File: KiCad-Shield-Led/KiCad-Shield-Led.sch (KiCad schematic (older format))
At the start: 16 parts, among them P1 Power, P2 Analog, P3 Digital, P4 Digital, P5 CONN_01X01, P6 CONN_01X01, P7 CONN_01X01, P8 CONN_01X01

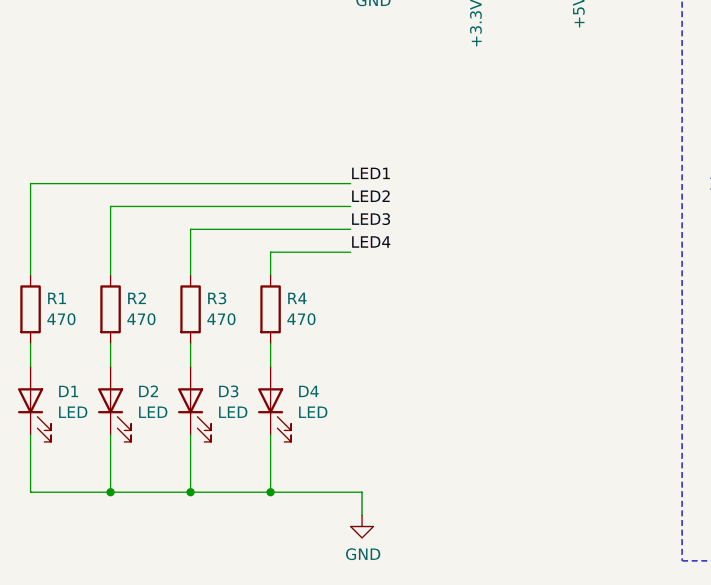
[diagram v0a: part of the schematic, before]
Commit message: Generation de la Netlist
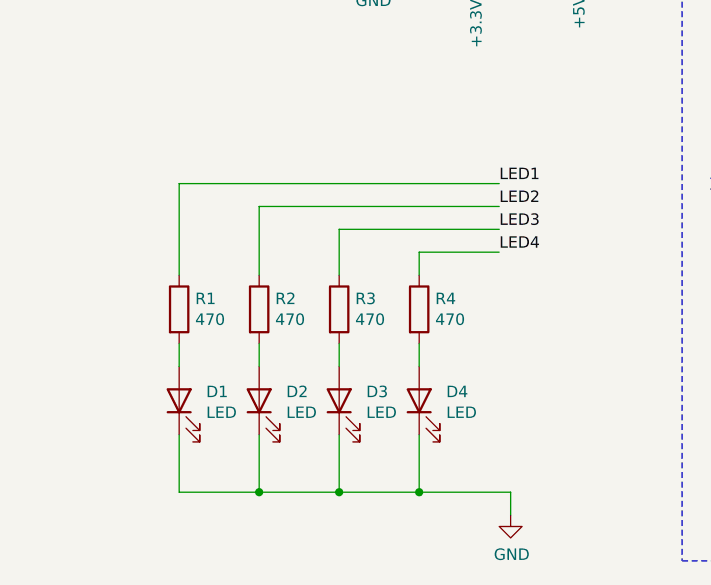
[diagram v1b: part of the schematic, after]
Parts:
- D1, D2, D3, D4: footprint (none) -> LED_THT:LED_D5.0mm
- R1, R2, R3, R4: footprint (none) -> Resistor_THT:R_Axial_DIN0207_L6.3mm_D2.5mm_P10.16mm_Horizontal
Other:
- moved on the sheet: D1, D2, D3, D4, R1, R2, R3, R4
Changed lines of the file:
@@
 L Device:LED D1
 U 1 1 5FC4CFF8
-P 5650 2750
-F 0 "D1" V 5689 2632 50  0000 R CNN
-F 1 "LED" V 5598 2632 50  0000 R CNN
-F 2 "" H 5650 2750 50  0001 C CNN
-F 3 "~" H 5650 2750 50  0001 C CNN
-	1    5650 2750
+P 6300 2750
+F 0 "D1" V 6339 2632 50  0000 R CNN
+F 1 "LED" V 6248 2632 50  0000 R CNN
+F 2 "LED_THT:LED_D5.0mm" H 6300 2750 50  0001 C CNN
+F 3 "~" H 6300 2750 50  0001 C CNN
+	1    6300 2750
 	0    -1   -1   0
 $EndComp
@@
 L Device:R R1
 U 1 1 5FC4E899
-P 5650 2350
-F 0 "R1" H 5720 2396 50  0000 L CNN
-F 1 "470" H 5720 2305 50  0000 L CNN
-F 2 "" V 5580 2350 50  0001 C CNN
-F 3 "~" H 5650 2350 50  0001 C CNN
-	1    5650 2350
+P 6300 2350
+F 0 "R1" H 6370 2396 50  0000 L CNN
+F 1 "470" H 6370 2305 50  0000 L CNN
+F 2 "Resistor_THT:R_Axial_DIN0207_L6.3mm_D2.5mm_P10.16mm_Horizontal" V 6230 2350 50  0001 C CNN
+F 3 "~" H 6300 2350 50  0001 C CNN
+	1    6300 2350
 	1    0    0    -1
 $EndComp
 Wire Wire Line
-	5650 2500 5650 2600
+	6300 2500 6300 2600
 Wire Wire Line
-	5650 2900 5650 3150
+	6300 2900 6300 3150
 Wire Wire Line
-	5650 3150 6000 3150
+	6300 3150 6650 3150
 Wire Wire Line
-	7100 3150 7100 3250
+	7750 3150 7750 3250
 $Comp
 L Device:LED D2
 U 1 1 5FC5721B
-P 6000 2750
-F 0 "D2" V 6039 2632 50  0000 R CNN
-F 1 "LED" V 5948 2632 50  0000 R CNN
-F 2 "" H 6000 2750 50  0001 C CNN
-F 3 "~" H 6000 2750 50  0001 C CNN
-	1    6000 2750
+P 6650 2750
+F 0 "D2" V 6689 2632 50  0000 R CNN
+F 1 "LED" V 6598 2632 50  0000 R CNN
+F 2 "LED_THT:LED_D5.0mm" H 6650 2750 50  0001 C CNN
+F 3 "~" H 6650 2750 50  0001 C CNN
+	1    6650 2750
 	0    -1   -1   0
 $EndComp
@@
 L Device:R R2
 U 1 1 5FC5738B
-P 6000 2350
-F 0 "R2" H 6070 2396 50  0000 L CNN
-F 1 "470" H 6070 2305 50  0000 L CNN
-F 2 "" V 5930 2350 50  0001 C CNN
-F 3 "~" H 6000 2350 50  0001 C CNN
-	1    6000 2350
+P 6650 2350
+F 0 "R2" H 6720 2396 50  0000 L CNN
+F 1 "470" H 6720 2305 50  0000 L CNN
+F 2 "Resistor_THT:R_Axial_DIN0207_L6.3mm_D2.5mm_P10.16mm_Horizontal" V 6580 2350 50  0001 C CNN
+F 3 "~" H 6650 2350 50  0001 C CNN
+	1    6650 2350
 	1    0    0    -1
 $EndComp
 Wire Wire Line
-	6000 2500 6000 2600
+	6650 2500 6650 2600
 Wire Wire Line
-	6000 2900 6000 3150
-Connection ~ 6000 3150
+	6650 2900 6650 3150
+Connection ~ 6650 3150
 Wire Wire Line
-	6000 3150 6350 3150
+	6650 3150 7000 3150
 $Comp
 L Device:LED D3
 U 1 1 5FC5A1AB
-P 6350 2750
-F 0 "D3" V 6389 2632 50  0000 R CNN
-F 1 "LED" V 6298 2632 50  0000 R CNN
-F 2 "" H 6350 2750 50  0001 C CNN
-F 3 "~" H 6350 2750 50  0001 C CNN
-	1    6350 2750
+P 7000 2750
+F 0 "D3" V 7039 2632 50  0000 R CNN
+F 1 "LED" V 6948 2632 50  0000 R CNN
+F 2 "LED_THT:LED_D5.0mm" H 7000 2750 50  0001 C CNN
+F 3 "~" H 7000 2750 50  0001 C CNN
+	1    7000 2750
 	0    -1   -1   0
 $EndComp
@@
 L Device:R R3
 U 1 1 5FC5A343
-P 6350 2350
-F 0 "R3" H 6420 2396 50  0000 L CNN
-F 1 "470" H 6420 2305 50  0000 L CNN
-F 2 "" V 6280 2350 50  0001 C CNN
-F 3 "~" H 6350 2350 50  0001 C CNN
-	1    6350 2350
+P 7000 2350
+F 0 "R3" H 7070 2396 50  0000 L CNN
+F 1 "470" H 7070 2305 50  0000 L CNN
+F 2 "Resistor_THT:R_Axial_DIN0207_L6.3mm_D2.5mm_P10.16mm_Horizontal" V 6930 2350 50  0001 C CNN
+F 3 "~" H 7000 2350 50  0001 C CNN
+	1    7000 2350
 	1    0    0    -1
 $EndComp
 Wire Wire Line
-	6350 2500 6350 2600
+	7000 2500 7000 2600
 Wire Wire Line
-	6350 2900 6350 3150
+	7000 2900 7000 3150
 $Comp
 L Device:LED D4
 U 1 1 5FC5A34F
-P 6700 2750
-F 0 "D4" V 6739 2632 50  0000 R CNN
-F 1 "LED" V 6648 2632 50  0000 R CNN
-F 2 "" H 6700 2750 50  0001 C CNN
-F 3 "~" H 6700 2750 50  0001 C CNN
-	1    6700 2750
+P 7350 2750
+F 0 "D4" V 7389 2632 50  0000 R CNN
+F 1 "LED" V 7298 2632 50  0000 R CNN
+F 2 "LED_THT:LED_D5.0mm" H 7350 2750 50  0001 C CNN
+F 3 "~" H 7350 2750 50  0001 C CNN
+	1    7350 2750
 	0    -1   -1   0
 $EndComp
@@
 L Device:R R4
 U 1 1 5FC5A359
-P 6700 2350
-F 0 "R4" H 6770 2396 50  0000 L CNN
-F 1 "470" H 6770 2305 50  0000 L CNN
-F 2 "" V 6630 2350 50  0001 C CNN
-F 3 "~" H 6700 2350 50  0001 C CNN
-	1    6700 2350
+P 7350 2350
+F 0 "R4" H 7420 2396 50  0000 L CNN
+F 1 "470" H 7420 2305 50  0000 L CNN
+F 2 "Resistor_THT:R_Axial_DIN0207_L6.3mm_D2.5mm_P10.16mm_Horizontal" V 7280 2350 50  0001 C CNN
+F 3 "~" H 7350 2350 50  0001 C CNN
+	1    7350 2350
 	1    0    0    -1
 $EndComp
 Wire Wire Line
-	6700 2500 6700 2600
+	7350 2500 7350 2600
 Wire Wire Line
-	6700 2900 6700 3150
-Connection ~ 6350 3150
+	7350 2900 7350 3150
+Connection ~ 7000 3150
 Wire Wire Line
-	6350 3150 6700 3150
-Connection ~ 6700 3150
+	7000 3150 7350 3150
+Connection ~ 7350 3150
 Wire Wire Line
-	6700 3150 7100 3150
+	7350 3150 7750 3150
 $Comp
 L power:GND #PWR05
 U 1 1 5FC5CA17
-P 7100 3250
-F 0 "#PWR05" H 7100 3000 50  0001 C CNN
-F 1 "GND" H 7105 3077 50  0000 C CNN
-F 2 "" H 7100 3250 50  0001 C CNN
-F 3 "" H 7100 3250 50  0001 C CNN
-	1    7100 3250
+P 7750 3250
+F 0 "#PWR05" H 7750 3000 50  0001 C CNN
+F 1 "GND" H 7755 3077 50  0000 C CNN
+F 2 "" H 7750 3250 50  0001 C CNN
+F 3 "" H 7750 3250 50  0001 C CNN
+	1    7750 3250
 	1    0    0    -1
 $EndComp
 Wire Wire Line
-	6700 2200 6700 2100
+	7350 2200 7350 2100
 Wire Wire Line
-	6700 2100 7050 2100
+	7350 2100 7700 2100
 Wire Wire Line
-	6350 2200 6350 2000
+	7000 2200 7000 2000
 Wire Wire Line
-	6350 2000 7050 2000
+	7000 2000 7700 2000
 Wire Wire Line
-	6000 1900 7050 1900
+	6650 1900 7700 1900
 Wire Wire Line
-	6000 1900 6000 2200
+	6650 1900 6650 2200
 Wire Wire Line
-	5650 2200 5650 1800
+	6300 2200 6300 1800
 Wire Wire Line
-	5650 1800 7050 1800
-Text Label 7050 1800 0    50   ~ 0
+	6300 1800 7700 1800
+Text Label 7700 1800 0    50   ~ 0
 LED1
-Text Label 7050 1900 0    50   ~ 0
+Text Label 7700 1900 0    50   ~ 0
 LED2
-Text Label 7050 2000 0    50   ~ 0
+Text Label 7700 2000 0    50   ~ 0
 LED3
-Text Label 7050 2100 0    50   ~ 0
+Text Label 7700 2100 0    50   ~ 0
 LED4
 Text Label 10550 1700 0    50   ~ 0
